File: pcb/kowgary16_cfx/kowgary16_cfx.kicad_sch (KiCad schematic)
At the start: 104 parts, among them J1 USB_C_Receptacle_USB2.0, SW1 SW_Push, SW10 SW_Push, SW11 SW_Push, SW12 SW_Push, SW13 SW_Push, SW14 SW_Push, SW15 SW_Push, SW16 SW_Push, SW17 SW_Push, SW18 SW_Push, SW19 SW_Push, SW2 SW_Push, SW20 SW_Push, SW21 SW_Push, SW22 SW_Push, SW23 SW_Push, SW24 SW_Push, SW25 SW_Push, SW26 SW_Push, SW27 SW_Push, SW28 SW_Push, SW29 SW_Push, SW3 SW_Push, SW30 SW_Push, SW31 SW_Push, SW32 SW_Push, SW33 SW_Push, SW34 SW_Push, SW35 SW_Push, SW36 SW_Push, SW37 SW_Push, SW38 SW_Push, SW39 SW_Push, SW4 SW_Push, SW40 SW_Push, SW5 SW_Push, SW6 SW_Push, SW7 SW_Push, SW8 SW_Push, SW9 SW_Push, U1 ATmega32U4-M, Y1 16MHz

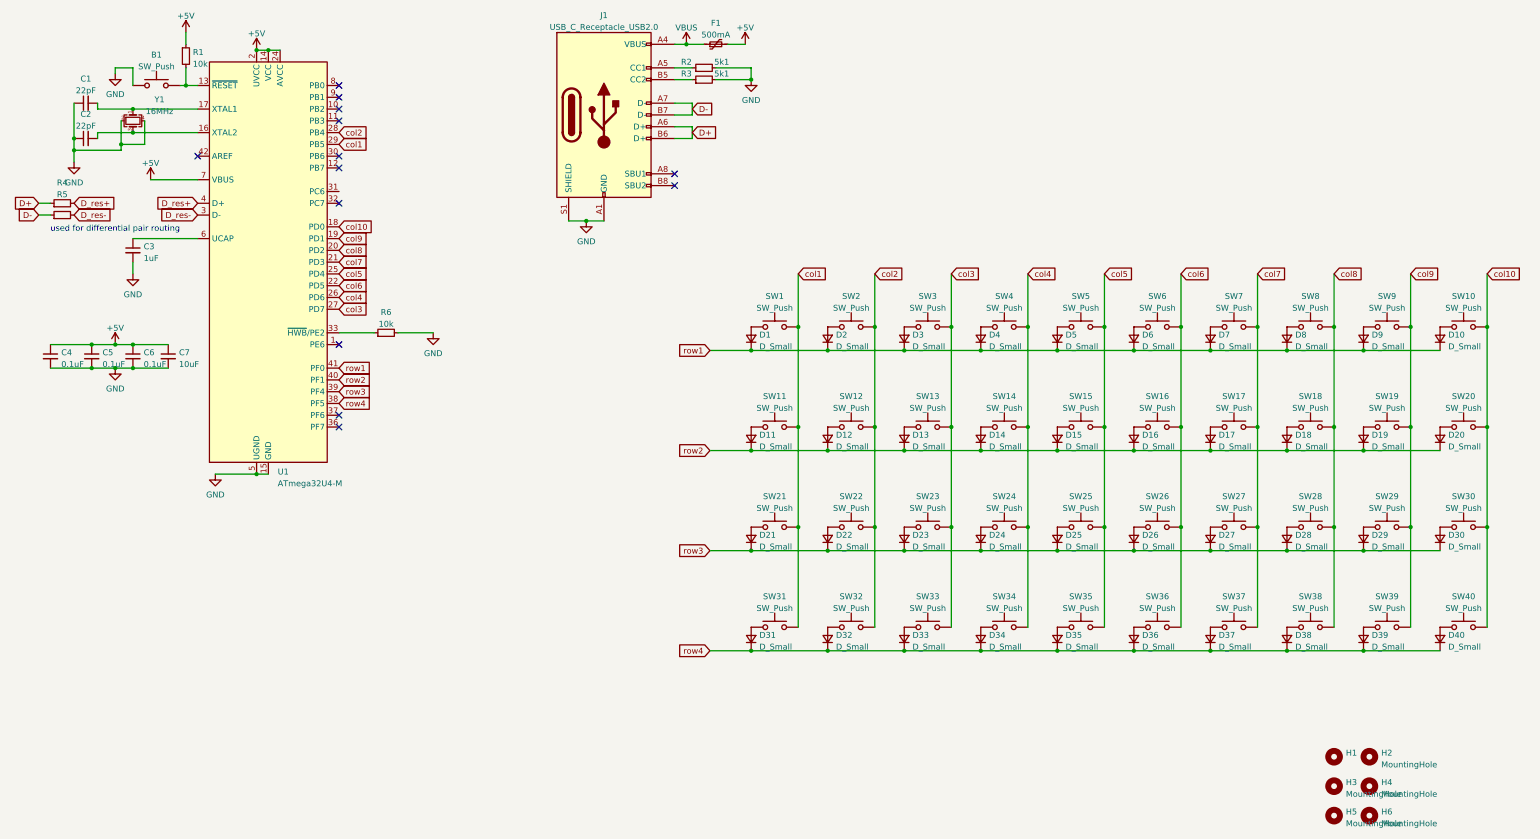
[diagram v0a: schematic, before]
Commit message: init commit
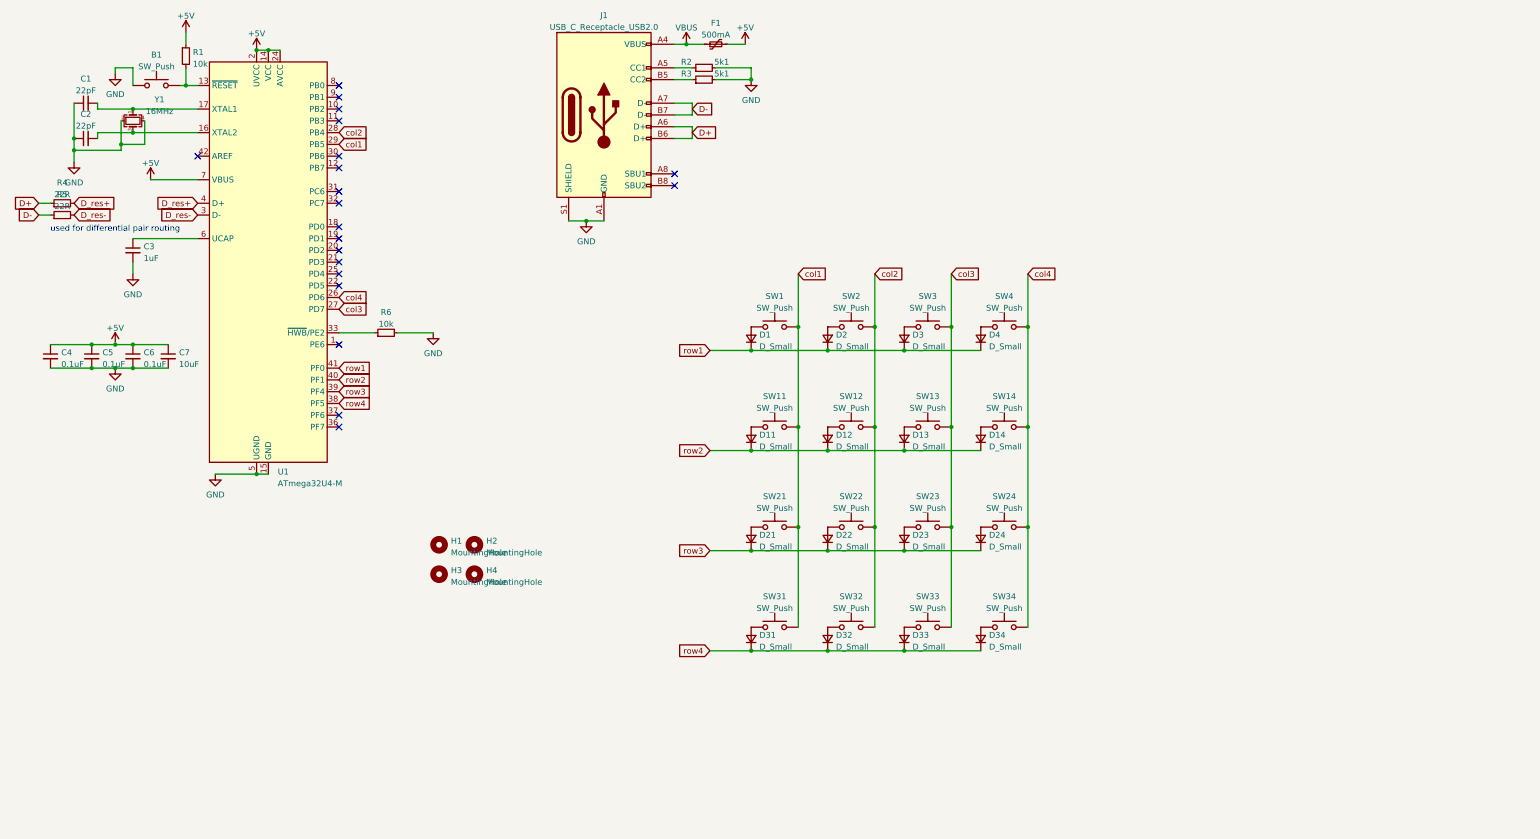
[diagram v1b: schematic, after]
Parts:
- removed D10, D15, D16, D17, D18, D19, D20, D25, D26, D27, D28, D29, D30, D35, D36, D37, D38, D39, D40, D5, D6, D7, D8, D9: D_Small, symbol Device:D_Small
- removed H5, H6: MountingHole, symbol Mechanical:MountingHole
- removed SW10, SW15, SW16, SW17, SW18, SW19, SW20, SW25, SW26, SW27, SW28, SW29, SW30, SW35, SW36, SW37, SW38, SW39, SW40, SW5, SW6, SW7, SW8, SW9: SW_Push, keyswitches:Kailh_socket_PG1350, symbol Switch:SW_Push
- C1, C2, C3, C4, C5, C6, C7: footprint (none) -> Capacitor_SMD:C_0402_1005Metric
- D1, D11, D12, D13, D14, D2, D21, D22, D23, D24, D3, D31, D32, D33, D34, D4: footprint (none) -> Diode_SMD:D_SOD-323
- F1: footprint (none) -> Fuse:Fuse_1206_3216Metric
- H1: value (none) -> MountingHole; footprint (none) -> MountingHole:MountingHole_2.2mm_M2_ISO7380
- H2, H3, H4: footprint (none) -> MountingHole:MountingHole_2.2mm_M2_ISO7380
- R1, R2, R3, R6: footprint (none) -> Resistor_SMD:R_0402_1005Metric
- R4, R5: value (none) -> 22R; footprint (none) -> Resistor_SMD:R_0402_1005Metric
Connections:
- net col10: no longer names the net of U1.18 (PD0)
- net col5: no longer names the net of U1.25 (PD4)
- net col6: no longer names the net of U1.22 (PD5)
- net col7: no longer names the net of U1.21 (PD3)
- net col8: no longer names the net of U1.20 (PD2)
- net col9: no longer names the net of U1.19 (PD1)
- no-connect marks 13 -> 20
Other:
- moved on the sheet: H1, H2, H3, H4
